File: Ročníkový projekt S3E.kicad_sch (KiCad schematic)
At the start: 40 parts, among them IC1 PIC18F47Q43-I_P, IC3 ULN2804A, IC5 MCP7940M-I_SN, J1 DG126-5.0-02P-14-00A, J2 - nastavení času, J3 + nastavení času, J7 TSW-105-07-G-S, J8 přepínání mezi číslicemi, Q1 DTA123JCAT116, Q2 DTA123JCAT116, Q3 DTA123JCAT116, Q4 DTA123JCAT116, Q5 DTA123JCAT116, Q6 DTA123JCAT116, Y1 32.768kHz

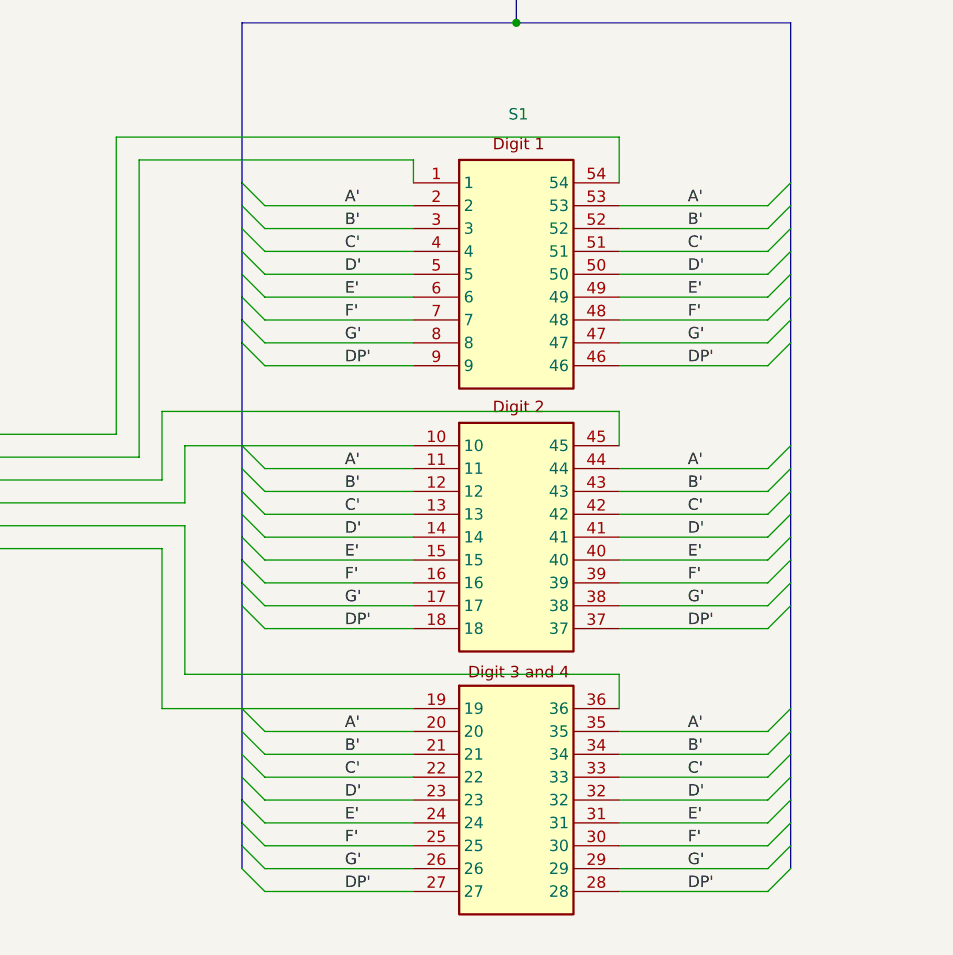
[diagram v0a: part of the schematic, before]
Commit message: backup update
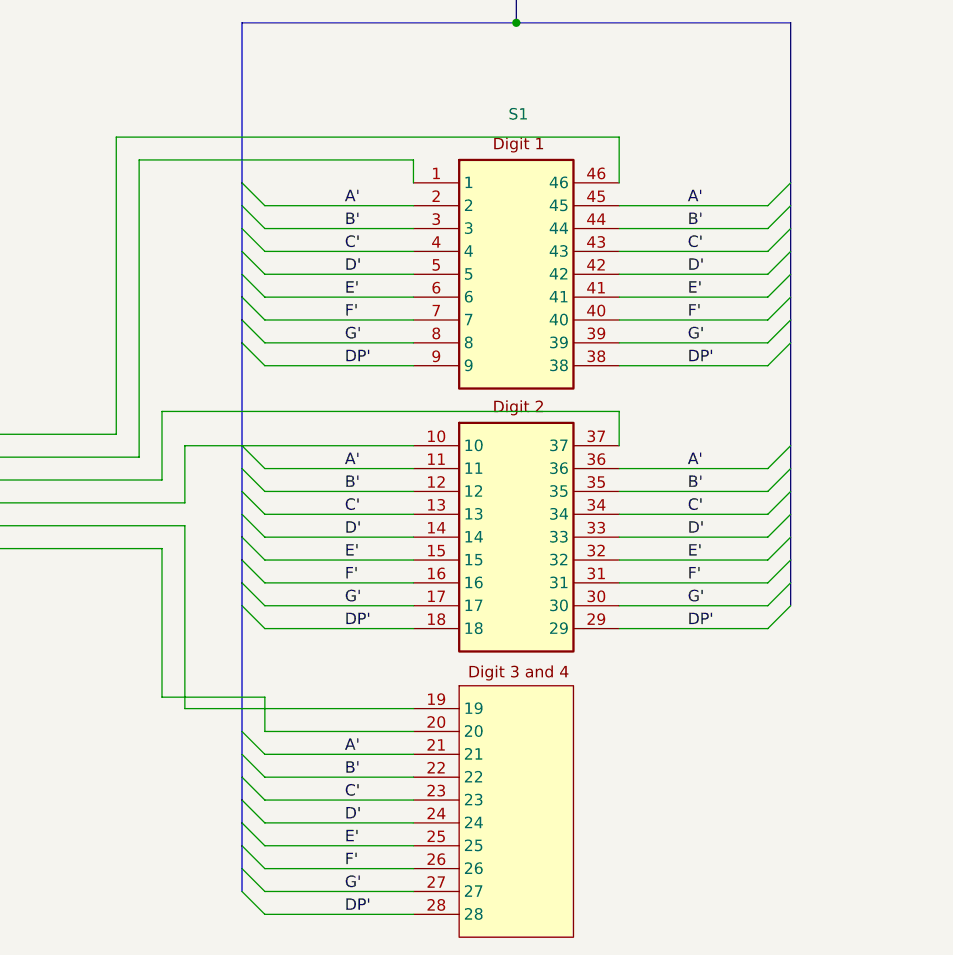
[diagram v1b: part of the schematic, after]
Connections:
- net A': now also S1.21, S1.36, S1.45; no longer S1.20, S1.35, S1.44, S1.53
- net B': now also S1.22, S1.35, S1.44; no longer S1.21, S1.34, S1.43, S1.52
- net C': now also S1.23, S1.34, S1.43; no longer S1.22, S1.33, S1.42, S1.51
- net D': now also S1.24, S1.33, S1.42; no longer S1.23, S1.32, S1.41, S1.50
- net DP': now also S1.29, S1.38; no longer S1.27, S1.37, S1.46
- net E': now also S1.25, S1.32, S1.41; no longer S1.24, S1.31, S1.40, S1.49
- net F': now also S1.26, S1.31, S1.40; no longer S1.25, S1.30, S1.39, S1.48
- net G': now also S1.27, S1.30, S1.39; no longer S1.26, S1.29, S1.38, S1.47
- net at Q6.1 (C): now also S1.20; no longer S1.19
- net at Q3.1 (C): now also S1.37; no longer S1.45
- net at Q5.1 (C): now also S1.19; no longer S1.36
- net at Q1.1 (C): now also S1.46; no longer S1.54

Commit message: backup update
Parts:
- IC5: footprint SamacSys_Parts:SOIC127P600X175-8N -> SOIC127P600X175-8N

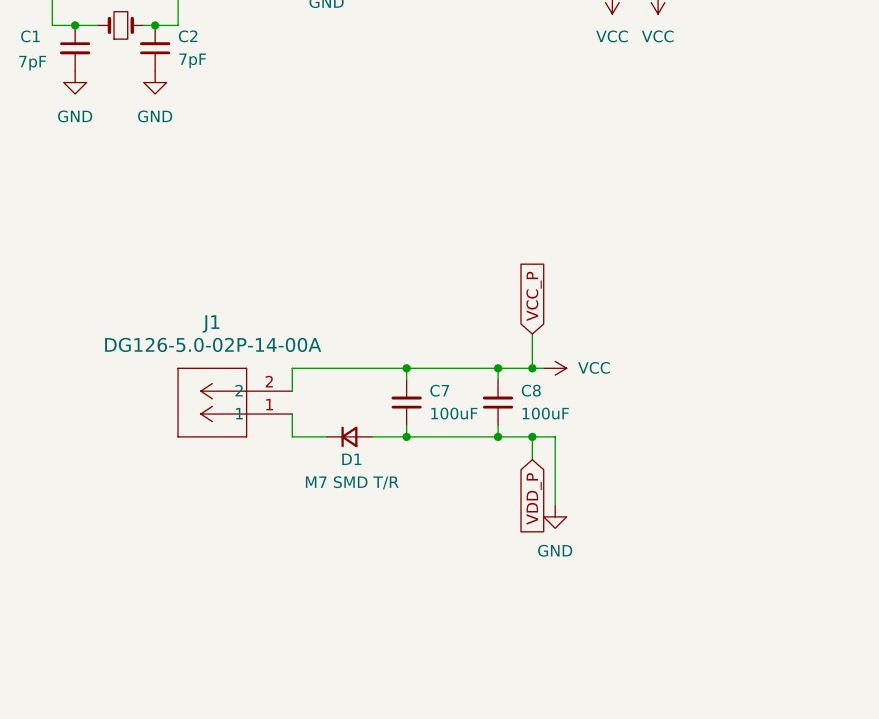
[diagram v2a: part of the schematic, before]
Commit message: backup update
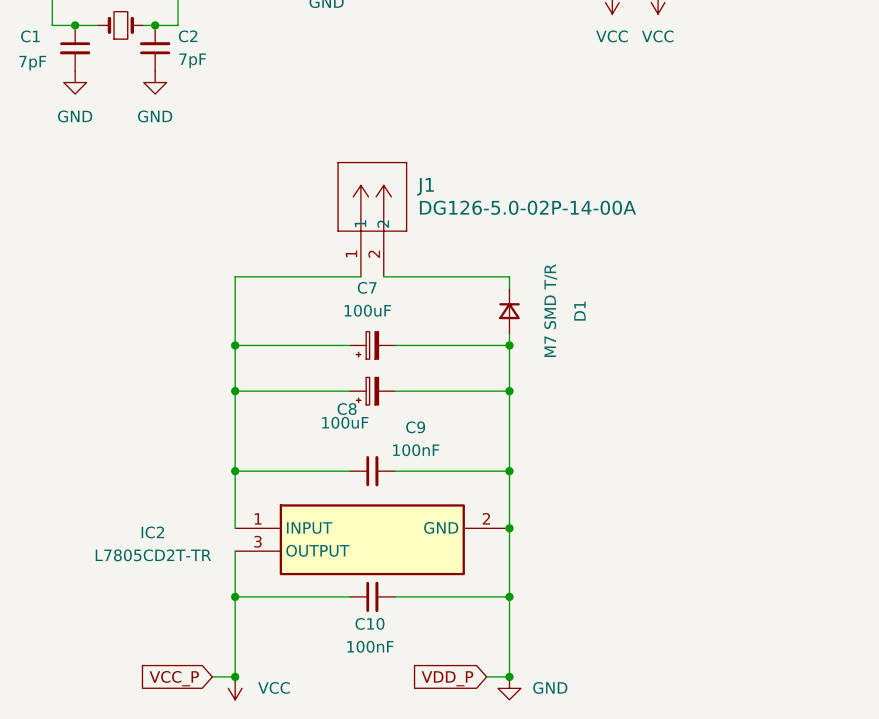
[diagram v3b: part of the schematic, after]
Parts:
- removed C7, C8: 100uF, Capacitor_THT:CP_Radial_D6.3mm_P2.50mm, symbol Device:C_Small
- added C10, C9: 100nF, Capacitor_SMD:C_1206_3216Metric_Pad1.33x1.80mm_HandSolder, symbol Device:C_Small
- added C7, C8: 100uF, Capacitor_THT:CP_Radial_D6.3mm_P2.50mm, symbol Device:C_Polarized_Small
- added IC2: L7805CD2T-TR, My parts:L7805CD2T, symbol My_parts:L7805CD2T-TR
- IC5: footprint SOIC127P600X175-8N -> My parts:SOIC127P600X175-8N
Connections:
- net GND: now also C10.2, C7.2, C8.2, C9.2, IC2.2 (GND)
- net VCC: now also C10.1, IC2.3 (OUTPUT); no longer J1.2
- net at J1.1: now also C7.1, C8.1, C9.1, IC2.1 (INPUT); no longer D1.1 (K)
- new net: D1.1 (K), J1.2
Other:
- moved on the sheet: D1, J1
